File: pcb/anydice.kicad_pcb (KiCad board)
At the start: 2 copper layers, 48 x 52 mm, 15 parts, among them J1 Conn_01x02, SW2 SW_SPST, U1 module_mpu6050, U2 XIAO ESP32C3, U3 ER_OLEDM0.91_1x-I2C, U4 TP4056-42-ESOP8

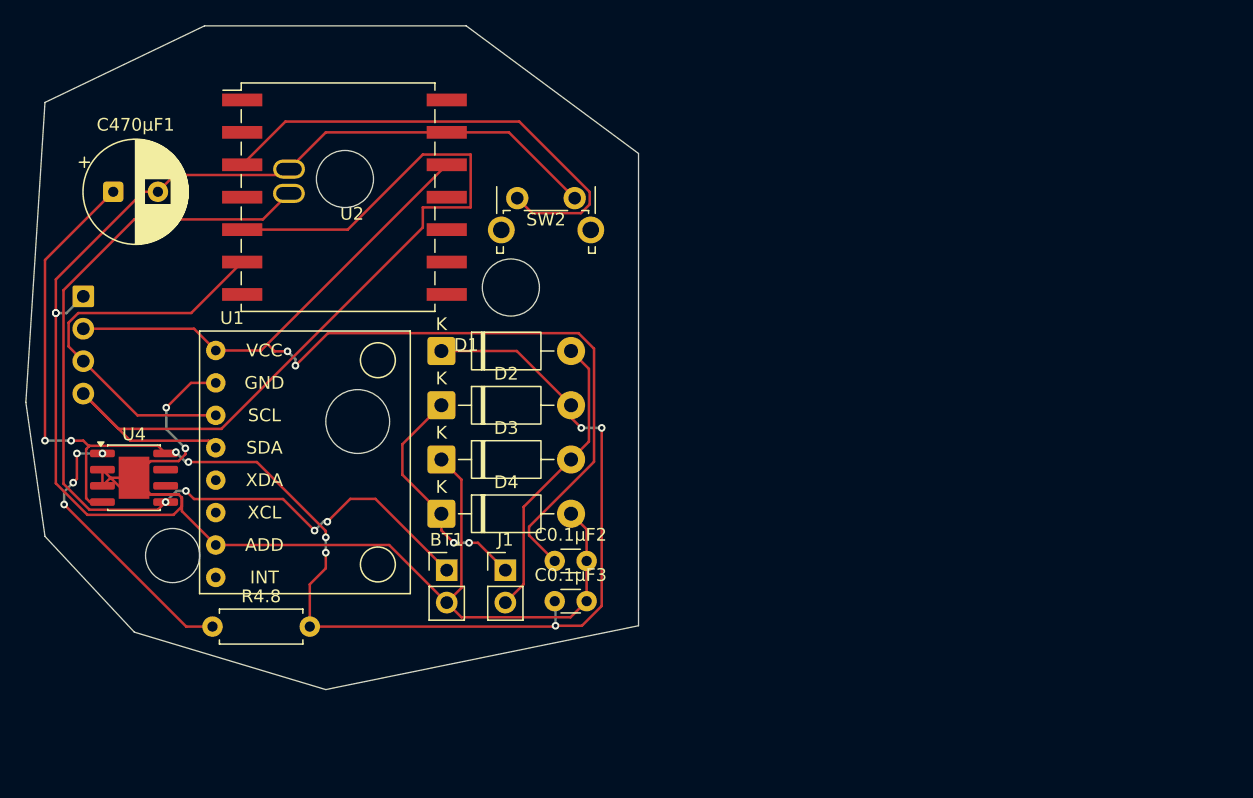
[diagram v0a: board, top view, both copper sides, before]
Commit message: added add the files and cadfiles
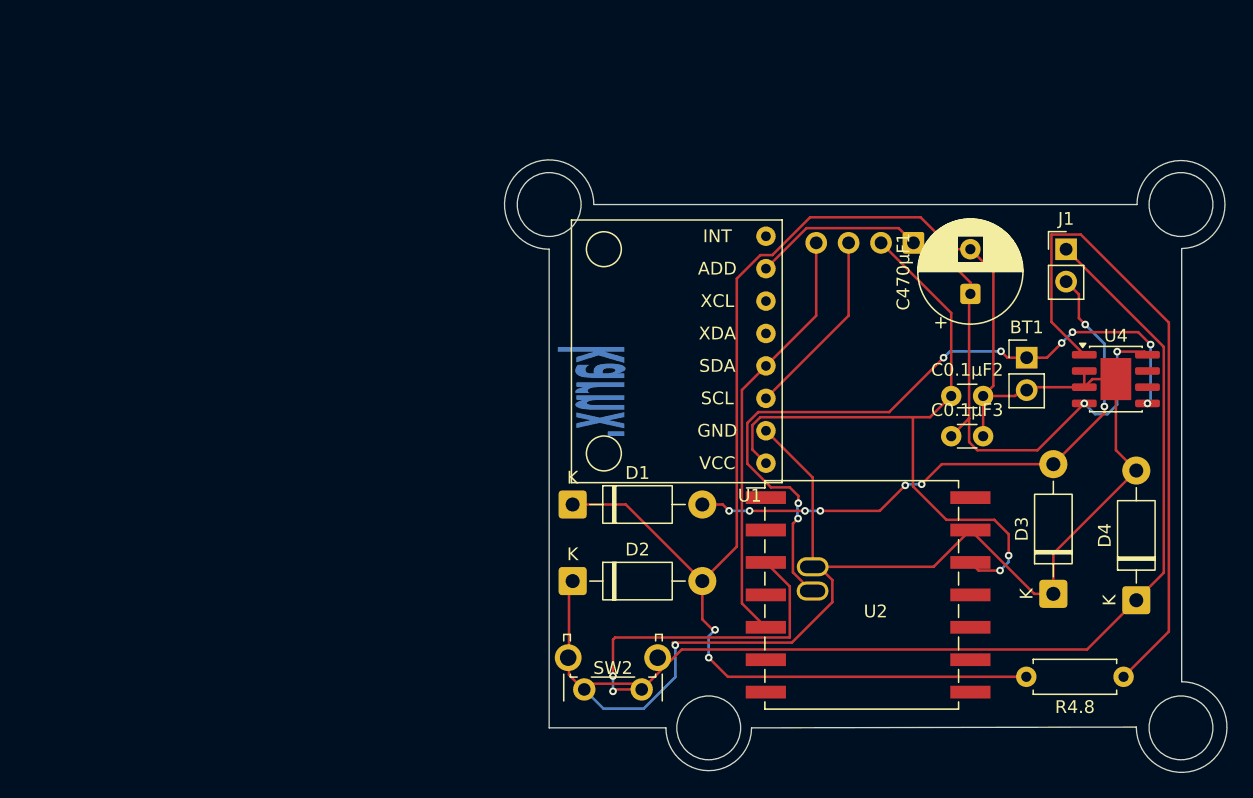
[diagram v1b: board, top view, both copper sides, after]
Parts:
- moved U4 77.3 mm to (210.9, 105.2)
- moved R4.8 71.5 mm to (211.5, 128.5), turned to 180 degrees
- moved C470µF1 67.6 mm to (199.5, 98.5), turned to 90 degrees
- moved U3 65.2 mm to (195.0, 94.5), turned to 180 degrees
- moved D4 54.9 mm to (212.5, 122.5), turned to 90 degrees
- moved U2 51.5 mm to (192.1, 123.9)
- moved U1 50.7 mm to (183.5, 94.0), turned to 180 degrees
- moved J1 50.6 mm to (207.0, 95.0)
- moved D3 49.1 mm to (206.0, 122.0), turned to 90 degrees
- moved BT1 48.4 mm to (203.9, 103.5)
- moved SW2 39.7 mm to (173.8, 129.5), turned to 180 degrees
- moved C0.1µF2 33.6 mm to (198.0, 106.5)
- moved C0.1µF3 33.6 mm to (198.0, 109.7)
- moved D2 17.2 mm to (168.3, 121.0)
- moved D1 15.8 mm to (168.3, 115.0)
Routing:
- net Net-(D2-K): track 18.6 -> 86.5 mm, vias 2 -> 0
- net Net-(U1-SDA): track 76.2 -> 33.3 mm
- net GND: track 163.4 -> 129.5 mm, vias 4 -> 1
- net Net-(U4-TEMP): track 22.0 -> 51.8 mm, vias 4 -> 0
- net /pwr: track 82.9 -> 54.4 mm
- net Net-(D1-A): track 23.0 -> 46.4 mm, vias 0 -> 8
- net Net-(U1-SCL): track 31.2 -> 14.9 mm
- net Net-(BT1-+): track 72.1 -> 56.7 mm, vias 4 -> 8
- net Net-(D1-K): track 115.4 -> 128.0 mm, vias 9 -> 6
- net Net-(SW2-A): track 38.3 -> 26.9 mm, vias 0 -> 2
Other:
- board size 48 x 52 mm -> 56.6 x 48 mm
